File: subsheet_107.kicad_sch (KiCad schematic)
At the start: 16 parts, among them T12 BDX54

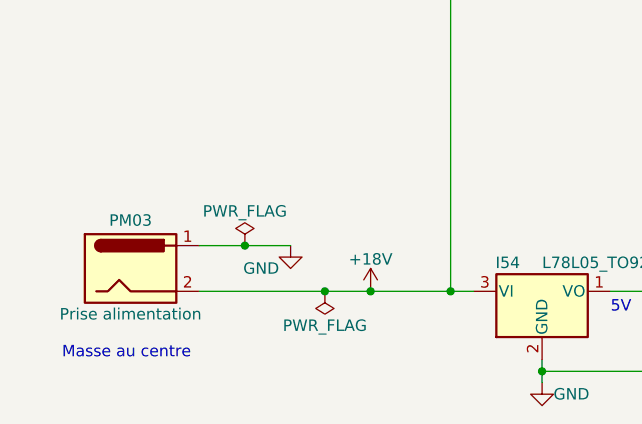
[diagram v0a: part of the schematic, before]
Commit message: Point de test 1
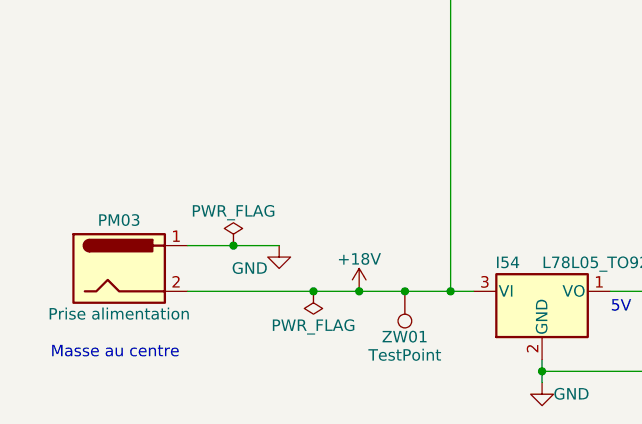
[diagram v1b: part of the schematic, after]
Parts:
- added ZW01: TestPoint, symbol Connector:TestPoint
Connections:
- net +15V: now also ZW01.1
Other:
- moved on the sheet: PM03
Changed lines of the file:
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@@
     (comment 4 "Reference : POP5001 501994-01")
   )
-  (junction (at 43.18 96.52) (diameter 0) (color 0 0 0 0)
+  (junction (at 60.96 101.6) (diameter 0) (color 0 0 0 0)
+  )
+  (junction (at 41.91 96.52) (diameter 0) (color 0 0 0 0)
   )
   (junction (at 137.16 59.69) (diameter 0) (color 0 0 0 0)
@@
   (junction (at 121.92 59.69) (diameter 0) (color 0 0 0 0)
   )
-  (junction (at 52.07 101.6) (diameter 0) (color 0 0 0 0)
-  )
-  (junction (at 57.15 101.6) (diameter 0) (color 0 0 0 0)
+  (junction (at 50.8 101.6) (diameter 0) (color 0 0 0 0)
+  )
+  (junction (at 55.88 101.6) (diameter 0) (color 0 0 0 0)
   )
   (junction (at 91.44 46.99) (diameter 0) (color 0 0 0 0)
@@
     (stroke (width 0) (type default) (color 0 0 0 0))
   )
-  (wire (pts (xy 38.1 96.52) (xy 43.18 96.52))
+  (wire (pts (xy 36.83 96.52) (xy 41.91 96.52))
     (stroke (width 0) (type default) (color 0 0 0 0))
   )
@@
     (stroke (width 0) (type default) (color 0 0 0 0))
   )
+  (wire (pts (xy 60.96 101.6) (xy 66.04 101.6))
+    (stroke (width 0) (type default) (color 0 0 0 0))
+  )
   (wire (pts (xy 71.12 46.99) (xy 76.2 46.99))
     (stroke (width 0) (type default) (color 0 0 0 0))
@@
     (stroke (width 0) (type default) (color 0 0 0 0))
   )
-  (wire (pts (xy 38.1 101.6) (xy 52.07 101.6))
+  (wire (pts (xy 36.83 101.6) (xy 50.8 101.6))
     (stroke (width 0) (type default) (color 0 0 0 0))
   )
@@
     (stroke (width 0) (type default) (color 0 0 0 0))
   )
-  (wire (pts (xy 43.18 96.52) (xy 48.26 96.52))
+  (wire (pts (xy 41.91 96.52) (xy 46.99 96.52))
     (stroke (width 0) (type default) (color 0 0 0 0))
   )
@@
     (stroke (width 0) (type default) (color 0 0 0 0))
   )
-  (wire (pts (xy 52.07 101.6) (xy 57.15 101.6))
+  (wire (pts (xy 50.8 101.6) (xy 55.88 101.6))
     (stroke (width 0) (type default) (color 0 0 0 0))
   )
@@
     (stroke (width 0) (type default) (color 0 0 0 0))
   )
-  (wire (pts (xy 57.15 101.6) (xy 66.04 101.6))
+  (wire (pts (xy 55.88 101.6) (xy 60.96 101.6))
     (stroke (width 0) (type default) (color 0 0 0 0))
   )
@@
     (stroke (width 0) (type default) (color 0 0 0 0))
   )
-  (text "Masse au centre" (at 22.86 109.22 0)
+  (text "Masse au centre" (at 21.59 109.22 0)
     (effects (font (size 1.27 1.27)) (justify left bottom))
   )
@@
     (pin "2")
   )
+  (symbol (lib_id "Connector:TestPoint") (at 60.96 101.6 180) (unit 1)
+    (in_bom yes) (on_board yes)
+    (property "Reference" "ZW01" (id 0) (at 60.96 106.68 0))
+    (property "Value" "TestPoint" (id 1) (at 60.96 108.712 0))
+    (property "Footprint" "" (id 2) (at 55.88 101.6 0)
+      (effects (font (size 1.27 1.27)) hide)
+    )
+    (property "Datasheet" "~" (id 3) (at 55.88 101.6 0)
+      (effects (font (size 1.27 1.27)) hide)
+    )
+    (pin "1")
+  )
   (symbol (lib_id "Device:C_Polarized_Small") (at 153.67 53.34 0) (unit 1)
     (in_bom yes) (on_board yes)
@@
     (pin "2")
   )
-  (symbol (lib_id "power-custom:+18V") (at 57.15 101.6 0) (unit 1)
-    (in_bom yes) (on_board yes)
-    (property "Reference" "#PWR?" (id 0) (at 57.15 105.41 0)
-      (effects (font (size 1.27 1.27)) hide)
-    )
-    (property "Value" "+18V" (id 1) (at 57.15 98.044 0))
-    (property "Footprint" "" (id 2) (at 57.15 101.6 0)
-      (effects (font (size 1.27 1.27)) hide)
-    )
-    (property "Datasheet" "" (id 3) (at 57.15 101.6 0)
+  (symbol (lib_id "power-custom:+18V") (at 55.88 101.6 0) (unit 1)
+    (in_bom yes) (on_board yes)
+    (property "Reference" "#PWR?" (id 0) (at 55.88 105.41 0)
+      (effects (font (size 1.27 1.27)) hide)
+    )
+    (property "Value" "+18V" (id 1) (at 55.88 98.044 0))
+    (property "Footprint" "" (id 2) (at 55.88 101.6 0)
+      (effects (font (size 1.27 1.27)) hide)
+    )
+    (property "Datasheet" "" (id 3) (at 55.88 101.6 0)
       (effects (font (size 1.27 1.27)) hide)
     )
@@
     (pin "2")
   )
-  (symbol (lib_id "power:GND") (at 48.26 96.52 0) (unit 1)
-    (in_bom yes) (on_board yes)
-    (property "Reference" "#PWR?" (id 0) (at 48.26 102.87 0)
-      (effects (font (size 1.27 1.27)) hide)
-    )
-    (property "Value" "GND" (id 1) (at 46.99 99.06 0)
+  (symbol (lib_id "power:GND") (at 46.99 96.52 0) (unit 1)
+    (in_bom yes) (on_board yes)
+    (property "Reference" "#PWR?" (id 0) (at 46.99 102.87 0)
+      (effects (font (size 1.27 1.27)) hide)
+    )
+    (property "Value" "GND" (id 1) (at 45.72 99.06 0)
       (effects (font (size 1.27 1.27)) (justify right))
     )
-    (property "Footprint" "" (id 2) (at 48.26 96.52 0)
-      (effects (font (size 1.27 1.27)) hide)
-    )
-    (property "Datasheet" "" (id 3) (at 48.26 96.52 0)
-      (effects (font (size 1.27 1.27)) hide)
-    )
-    (pin "1")
-  )
-  (symbol (lib_id "Connector:Jack-DC") (at 30.48 99.06 0) (unit 1)
-    (in_bom yes) (on_board yes)
-    (property "Reference" "PM03" (id 0) (at 30.48 93.726 0))
-    (property "Value" "Prise alimentation" (id 1) (at 30.48 104.14 0))
-    (property "Footprint" "" (id 2) (at 31.75 100.076 0)
-      (effects (font (size 1.27 1.27)) hide)
-    )
-    (property "Datasheet" "~" (id 3) (at 31.75 100.076 0)
+    (property "Footprint" "" (id 2) (at 46.99 96.52 0)
+      (effects (font (size 1.27 1.27)) hide)
+    )
+    (property "Datasheet" "" (id 3) (at 46.99 96.52 0)
+      (effects (font (size 1.27 1.27)) hide)
+    )
+    (pin "1")
+  )
+  (symbol (lib_id "Connector:Jack-DC") (at 29.21 99.06 0) (unit 1)
+    (in_bom yes) (on_board yes)
+    (property "Reference" "PM03" (id 0) (at 29.21 93.726 0))
+    (property "Value" "Prise alimentation" (id 1) (at 29.21 104.14 0))
+    (property "Footprint" "" (id 2) (at 30.48 100.076 0)
+      (effects (font (size 1.27 1.27)) hide)
+    )
+    (property "Datasheet" "~" (id 3) (at 30.48 100.076 0)
       (effects (font (size 1.27 1.27)) hide)
     )
@@
     (pin "1")
   )
-  (symbol (lib_id "power:PWR_FLAG") (at 43.18 96.52 0) (unit 1)
-    (in_bom yes) (on_board yes)
-    (property "Reference" "#FLG?" (id 0) (at 43.18 94.615 0)
-      (effects (font (size 1.27 1.27)) hide)
-    )
-    (property "Value" "PWR_FLAG" (id 1) (at 43.18 92.71 0))
-    (property "Footprint" "" (id 2) (at 43.18 96.52 0)
-      (effects (font (size 1.27 1.27)) hide)
-    )
-    (property "Datasheet" "~" (id 3) (at 43.18 96.52 0)
+  (symbol (lib_id "power:PWR_FLAG") (at 41.91 96.52 0) (unit 1)
+    (in_bom yes) (on_board yes)
+    (property "Reference" "#FLG?" (id 0) (at 41.91 94.615 0)
+      (effects (font (size 1.27 1.27)) hide)
+    )
+    (property "Value" "PWR_FLAG" (id 1) (at 41.91 92.71 0))
+    (property "Footprint" "" (id 2) (at 41.91 96.52 0)
+      (effects (font (size 1.27 1.27)) hide)
+    )
+    (property "Datasheet" "~" (id 3) (at 41.91 96.52 0)
       (effects (font (size 1.27 1.27)) hide)
     )
@@
     (pin "1")
   )
-  (symbol (lib_id "power:PWR_FLAG") (at 52.07 101.6 180) (unit 1)
-    (in_bom yes) (on_board yes)
-    (property "Reference" "#FLG?" (id 0) (at 52.07 103.505 0)
-      (effects (font (size 1.27 1.27)) hide)
-    )
-    (property "Value" "PWR_FLAG" (id 1) (at 52.07 105.41 0))
-    (property "Footprint" "" (id 2) (at 52.07 101.6 0)
-      (effects (font (size 1.27 1.27)) hide)
-    )
-    (property "Datasheet" "~" (id 3) (at 52.07 101.6 0)
-      (effects (font (size 1.27 1.27)) hide)
-    )
+  (symbol (lib_id "power:PWR_FLAG") (at 50.8 101.6 180) (unit 1)
+    (in_bom yes) (on_board yes)
+    (property "Reference" "#FLG?" (id 0) (at 50.8 103.505 0)
+      (effects (font (size 1.27 1.27)) hide)
+    )
+    (property "Value" "PWR_FLAG" (id 1) (at 50.8 105.41 0))
+    (property "Footprint" "" (id 2) (at 50.8 101.6 0)
+      (effects (font (size 1.27 1.27)) hide)
+    )
+    (property "Datasheet" "~" (id 3) (at 50.8 101.6 0)
+      (effects (font (size 1.27 1.27)) hide)
+    )
